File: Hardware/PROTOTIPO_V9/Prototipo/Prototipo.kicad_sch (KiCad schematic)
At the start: 1 part, among them U1 YAAJ_BluePill_Part_Like_SWD_B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

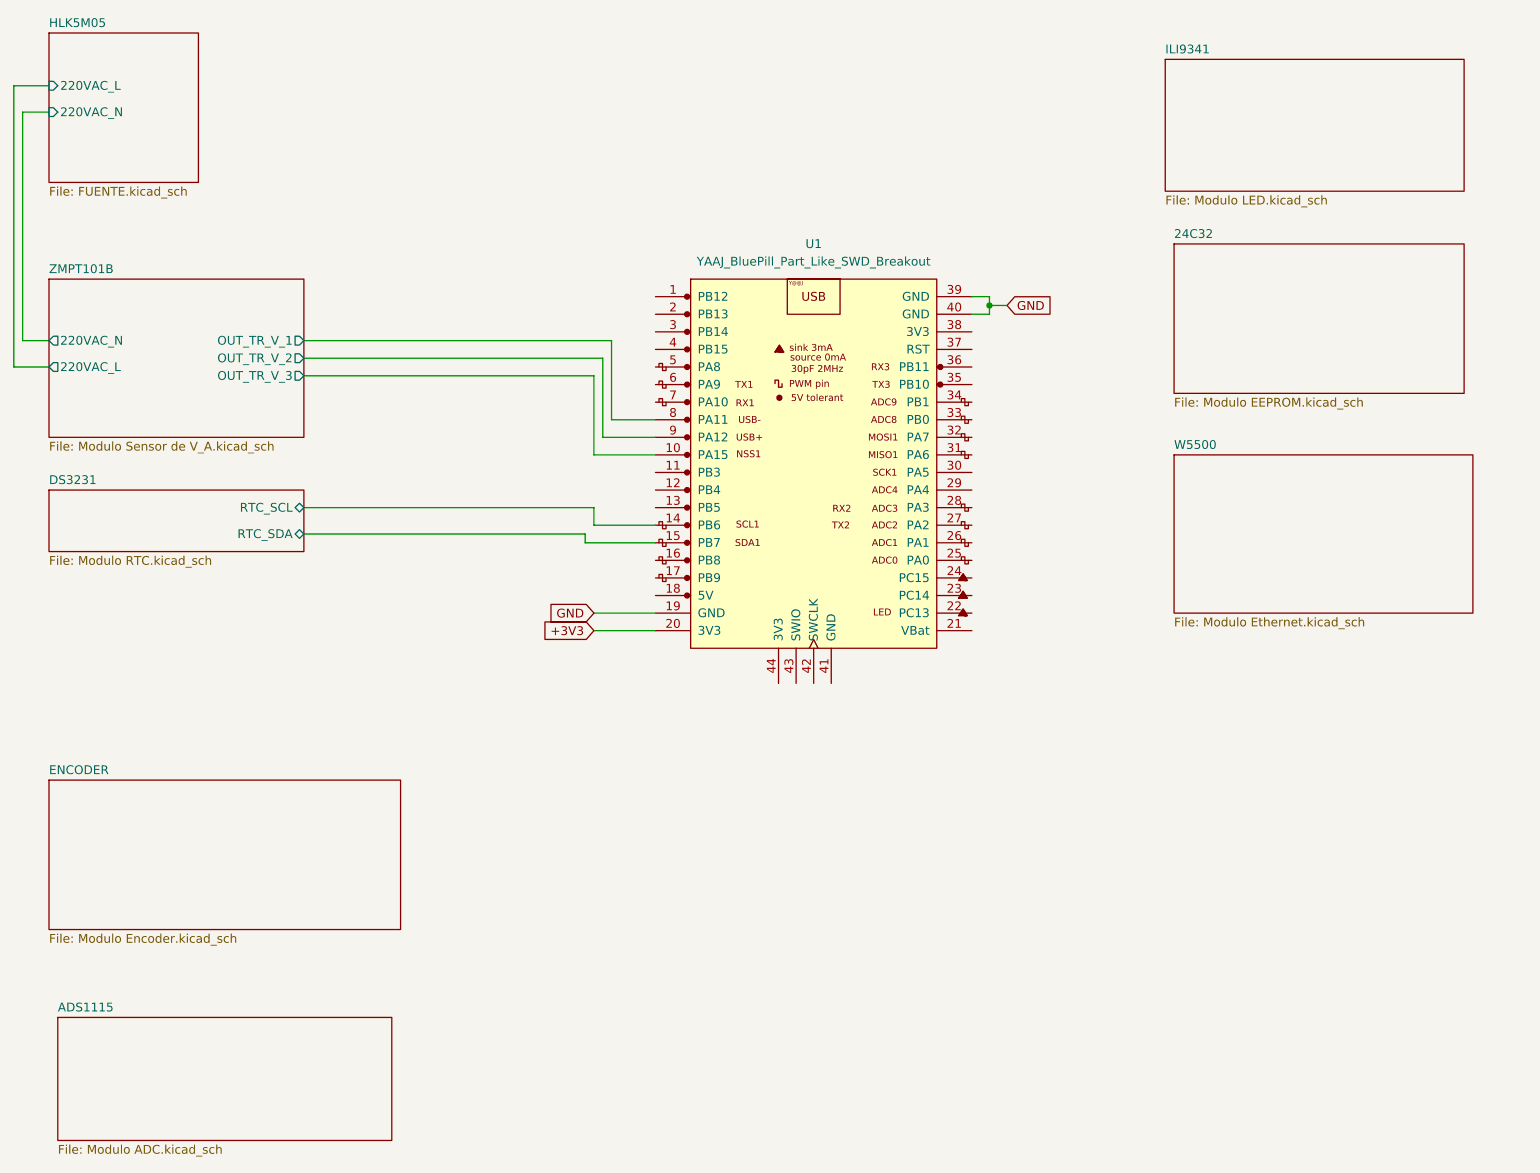
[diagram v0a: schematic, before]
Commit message: Esquematico Encoder
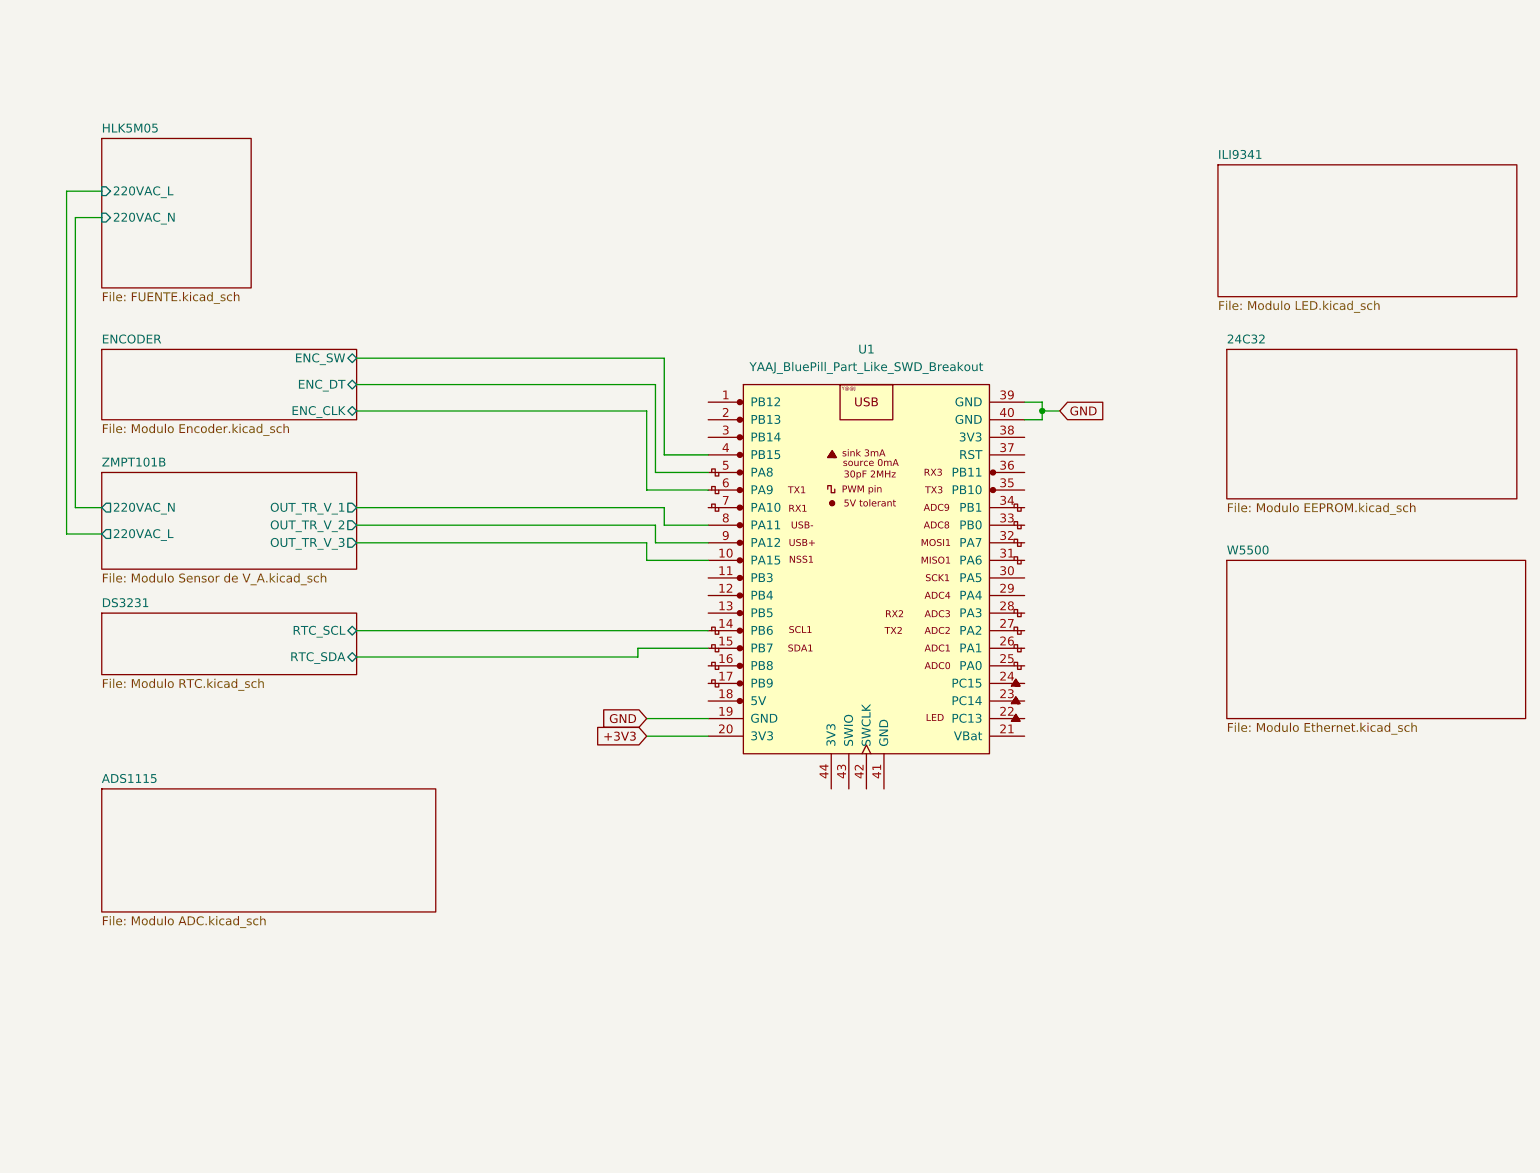
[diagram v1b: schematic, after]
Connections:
- net ENCODER/ENC_SW: now reaches U1.4 (PB15)
- net ENCODER/ENC_DT: now reaches U1.5 (PA8)
- net ENCODER/ENC_CLK: now reaches U1.6 (PA9)
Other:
- sheet ENCODER ports: added ENC_CLK, ENC_DT, ENC_SW; removed none
- moved on the sheet: U1
